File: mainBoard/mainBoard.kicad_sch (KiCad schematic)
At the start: 69 parts, among them J3 Conn_02x24_Odd_Even, Q10 FDV303N, Q11 FDV303N, Q12 FDV303N, Q13 FDV303N, Q14 FDV303N, Q15 FDV303N, Q16 FDV303N, Q17 FDV303N, Q2 FDV303N, Q3 FDV303N, Q4 FDV303N, Q5 FDV303N, Q6 FDV303N, Q7 FDV303N, Q8 FDV303N, Q9 FDV303N, U1 W25Q128JVS, U3 TLC59283DBQR, U4 TLC59283DBQR, U6 DRV5033FAxDBZ, U8 RP2040, Y2 ABM8-272-T3

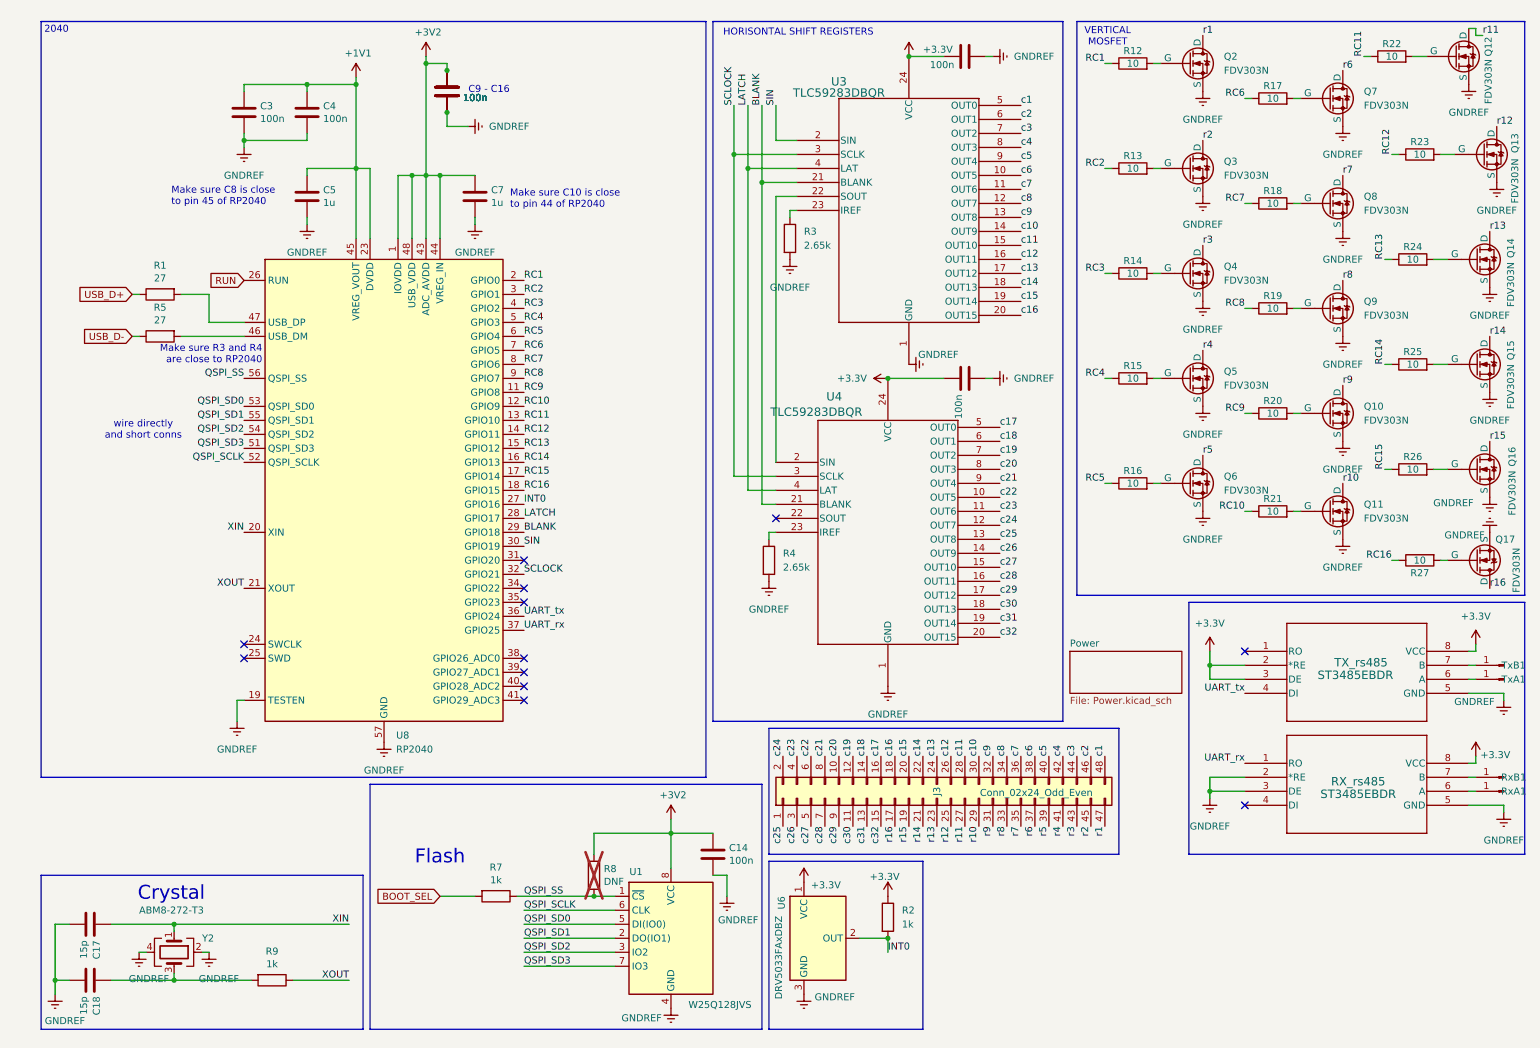
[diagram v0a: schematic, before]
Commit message: getting ready for another review
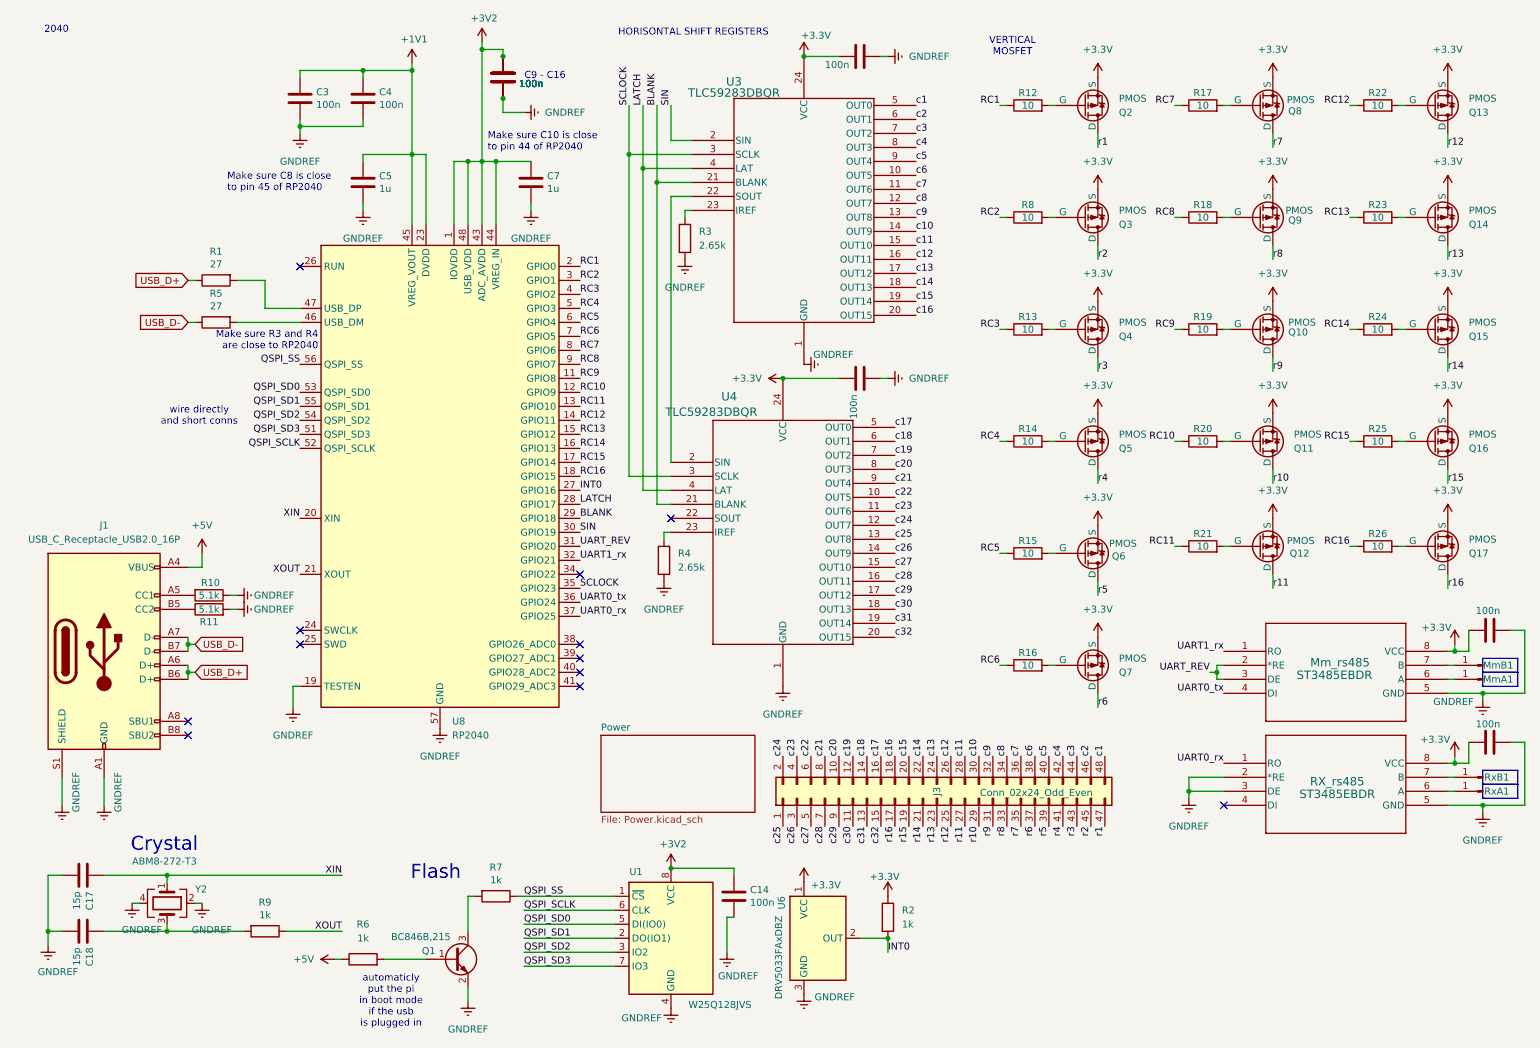
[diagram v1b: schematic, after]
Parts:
- removed Q10, Q11, Q12, Q13, Q14, Q15, Q16, Q17, Q2, Q3, Q4, Q5, Q6, Q7, Q8, Q9: FDV303N, Package_TO_SOT_SMD:SOT-23, symbol Simulation_SPICE:NMOS
- removed R27: 10, Resistor_SMD:R_0402_1005Metric, symbol Device:R
- added C15, C22: 100n, Capacitor_SMD:C_0402_1005Metric, symbol Device:C
- added J1: USB_C_Receptacle_USB2.0_16P, Connector_USB:USB_C_Receptacle_G-Switch_GT-USB-7010ASV, symbol Connector:USB_C_Receptacle_USB2.0_16P
- added Q1: BC846B,215, Package_TO_SOT_SMD:SOT-323_SC-70, symbol Transistor_BJT:2SC4213
- added Q10, Q11, Q12, Q13, Q14, Q15, Q16, Q17, Q2, Q3, Q4, Q5, Q6, Q7, Q8, Q9: PMOS, Package_TO_SOT_SMD:SOT-416, symbol Simulation_SPICE:PMOS
- added R10, R11: 5.1k, Resistor_SMD:R_0402_1005Metric, symbol Device:R
- added R6: 1k, Resistor_SMD:R_0402_1005Metric, symbol Device:R
- R8: value DNF -> 10; LCSC PN (none) -> C100206; MPN (none) -> CR0402FF10R0G; Manufacturer (none) -> LIZ Elec; now fitted
- U1: footprint Package_SO:SOIC-8_7.5x5.85mm_P1.27mm -> Package_DFN_QFN:WFDFPN-8-1EP_3x2mm_P0.5mm_EP1.25x1.35mm
- renumbered TxA1 to MmA1, TxB1 to MmB1, TX_rs485 to Mm_rs485
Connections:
- net +3.3V: now also C15.2, C22.2, Q10.3 (S), Q11.3 (S), Q12.3 (S), Q13.3 (S), Q14.3 (S), Q15.3 (S), Q16.3 (S), Q17.3 (S), Q2.3 (S), Q3.3 (S), Q4.3 (S), Q5.3 (S), Q6.3 (S), Q7.3 (S), Q8.3 (S), Q9.3 (S); no longer Mm_rs485.2 (*RE), Mm_rs485.3 (DE)
- net +3V2: no longer R8.1
- net GNDREF: now also C15.1, C22.1, J1.A1 (GND), J1.A12 (GND), J1.B1 (GND), J1.B12 (GND), J1.S1 (SHIELD), Q1.2 (E), R10.1, R11.2
- net QSPI_SS: no longer R8.2
- net RC10: now also R20.1; no longer R21.1
- net RC11: now also R21.1; no longer R22.1
- net RC12: now also R22.1; no longer R23.1
- net RC13: now also R23.1; no longer R24.1
- net RC14: now also R24.1; no longer R25.1
- net RC15: now also R25.1; no longer R26.1
- net RC16: now also R26.1
- net RC2: now also R8.1; no longer R13.1
- net RC3: now also R13.1; no longer R14.1
- net RC4: now also R14.1; no longer R15.1
- net RC5: now also R15.1; no longer R16.1
- net RC6: now also R16.1; no longer R17.1
- net RC7: now also R17.1; no longer R18.1
- net RC8: now also R18.1; no longer R19.1
- net RC9: now also R19.1; no longer R20.1
- net SCLOCK: now also U8.35 (GPIO23); no longer U8.32 (GPIO21)
- net USB_D+: now also J1.A6 (D+), J1.B6 (D+)
- net USB_D-: now also J1.A7 (D-), J1.B7 (D-)
- net r1: now also Q2.1 (D)
- net r10: now also Q11.1 (D)
- net r11: now also Q12.1 (D)
- net r12: now also Q13.1 (D)
- net r13: now also Q14.1 (D)
- net r14: now also Q15.1 (D)
- net r15: now also Q16.1 (D)
- net r16: now also Q17.1 (D)
- net r2: now also Q3.1 (D)
- net r3: now also Q4.1 (D)
- net r4: now also Q5.1 (D)
- net r5: now also Q6.1 (D)
- net r6: now also Q7.1 (D)
- net r7: now also Q8.1 (D)
- net r8: now also Q9.1 (D)
- net r9: now also Q10.1 (D)
- net at R18.2: now also Q9.2 (G)
- net at R26.2: now also Q17.2 (G)
- net at R24.2: now also Q15.2 (G)
- net at R16.2: now also Q7.2 (G)
- net at R22.2: now also Q13.2 (G)
- net at R21.2: now also Q12.2 (G)
- net at R20.2: now also Q11.2 (G)
- net at R25.2: now also Q16.2 (G)
- net at R15.2: now also Q6.2 (G)
- net at R12.2: now also Q2.2 (G)
- net UART_REV: now reaches U8.31 (GPIO20)
- net UART_REV: now also Mm_rs485.2 (*RE), Mm_rs485.3 (DE)
- net at R19.2: now also Q10.2 (G)
- net at R17.2: now also Q8.2 (G)
- net UART1_rx: now reaches Mm_rs485.1 (RO)
- net UART1_rx: now also U8.32 (GPIO21)
- net at R23.2: now also Q14.2 (G)
- net at R13.2: now also Q4.2 (G)
- net at R14.2: now also Q5.2 (G)
- net BOOT_SEL: no longer names the net of R7.2
- net BOOT_SEL: now also Q1.3 (C)
- net RUN: no longer names the net of U8.26 (RUN)
- net UART_rx renamed UART0_rx
- net UART_tx renamed UART0_tx
- new net: Q3.2 (G), R8.2
- new net: J1.B5 (CC2), R11.1
- new net: Q1.1 (B), R6.2
- new net: J1.A5 (CC1), R10.2
- new net +5V: J1.A4 (VBUS), J1.A9 (VBUS), J1.B4 (VBUS), J1.B9 (VBUS), R6.1
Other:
- note added: "automaticly put the pi in boot mode if the usb is plugged in"
- moved on the sheet: C14, C17, C18, C3, C4, C5, C7, MmA1, MmB1, Mm_rs485, R1, R12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
